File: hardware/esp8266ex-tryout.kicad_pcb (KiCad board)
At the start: 2 copper layers, 20 parts, among them U1 ESP8266EX, U2 W25Q32JVSSIQ, Y1 O_26M,3225

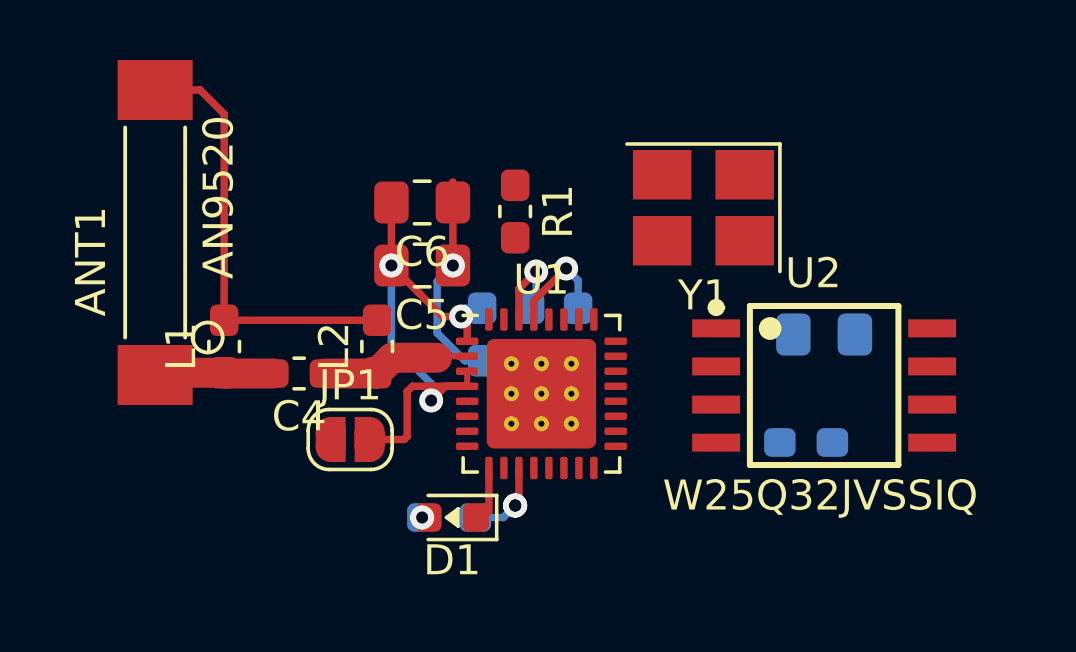
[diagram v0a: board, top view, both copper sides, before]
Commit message: update,
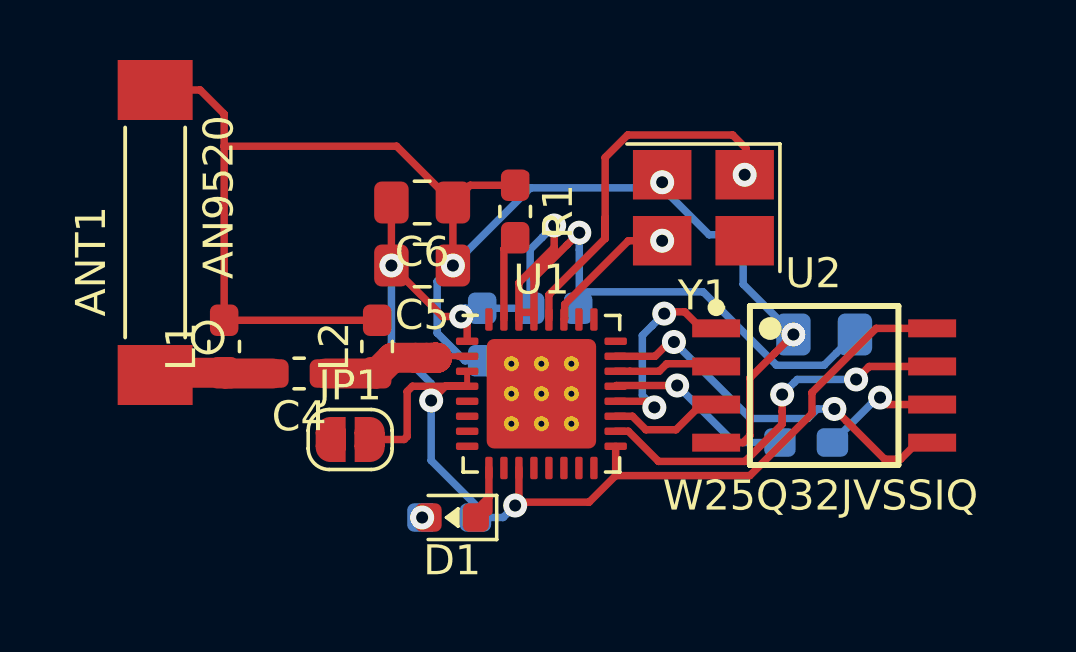
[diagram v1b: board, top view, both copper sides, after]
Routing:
- net Vesp8266: track 28.3 -> 69.6 mm, vias 7 -> 6
- net GND: track 34.5 -> 66.9 mm, vias 1 -> 3
- net Net-(C1-Pad2): track 0.00 -> 14.4 mm, vias 0 -> 1
- net /SD_D2: track 0.00 -> 12.9 mm, vias 0 -> 2
- net /SD_D1: track 0.00 -> 12.9 mm, vias 0 -> 2
- net /SD_CMD: track 0.00 -> 6.95 mm, vias 0 -> 2
- net Net-(R2-Pad2): track 0.00 -> 6.27 mm, vias 0 -> 1
- net Net-(C2-Pad2): track 0.00 -> 4.84 mm, vias 0 -> 1
- net /SD_CLK: track 0.00 -> 4.04 mm, vias 0 -> 1
- net /SD_D3: track 0.00 -> 3.88 mm
- net /SD_D0: track 0.00 -> 3.49 mm
- net Net-(R1-Pad2): track 0.00 -> 2.88 mm
- net /GPIO14: track 1.46 -> 2.32 mm
